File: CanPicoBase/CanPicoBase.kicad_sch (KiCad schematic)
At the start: 17 parts, among them J1 3.50 CBUS, J2 5V select, J3 Grove 2mm, J4 Conn_01x20_Male, J5 Conn_01x20_Male, Q1 DMG2305UX-7, U1 AMS1117-5.0, U2 AMS1117-3.3, U3 Pico

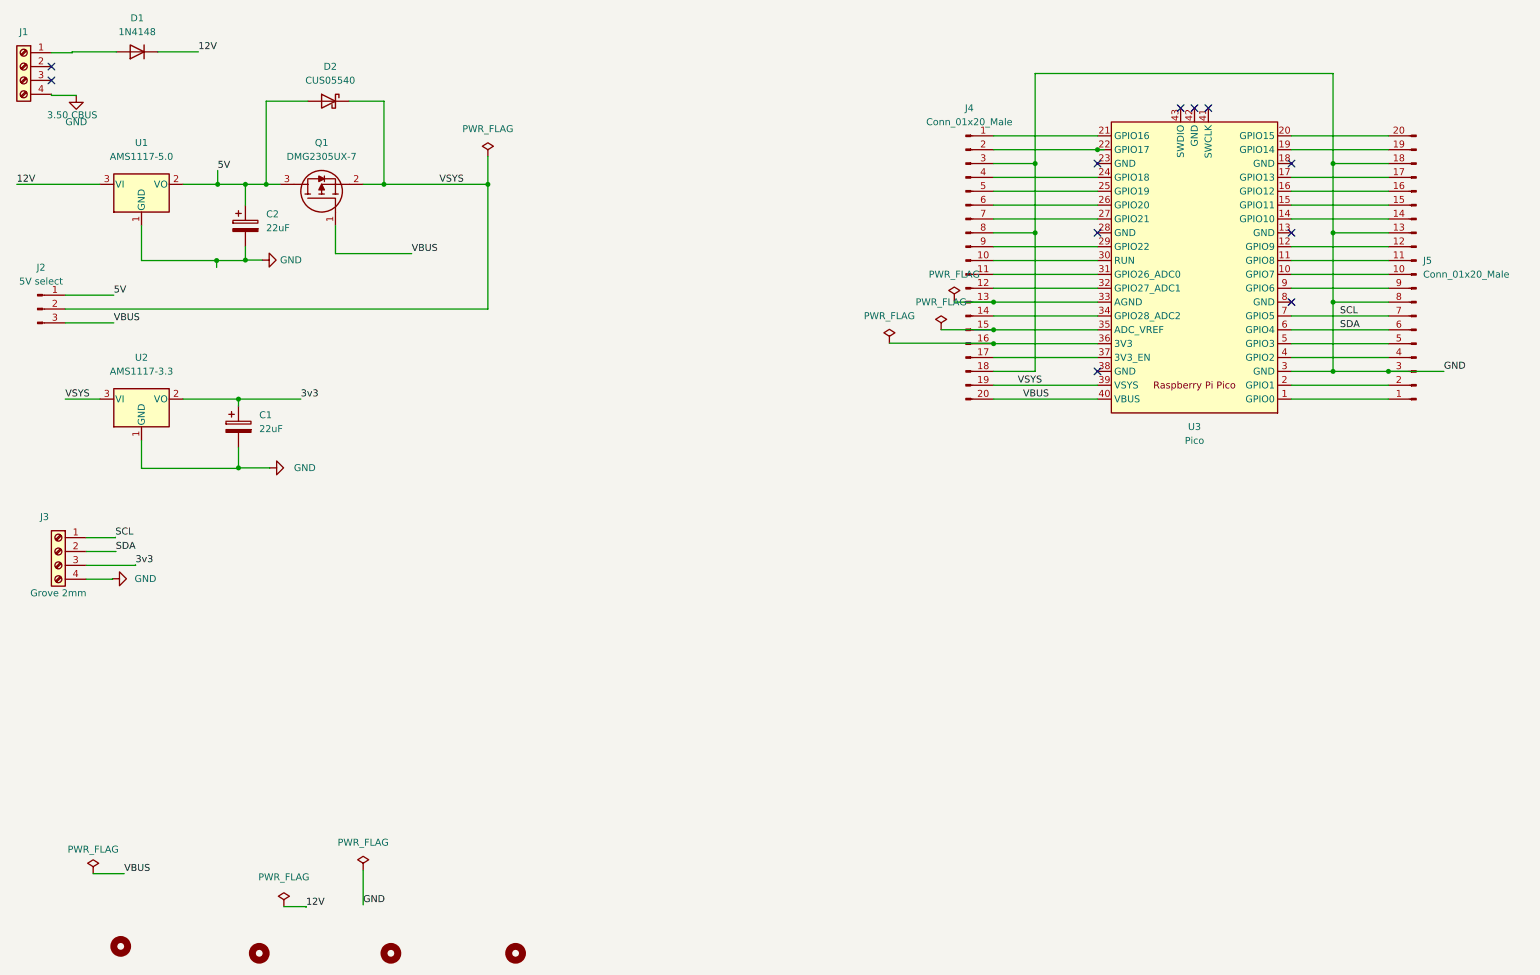
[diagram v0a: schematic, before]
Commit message: 08/09/25 13:36 Titan.local
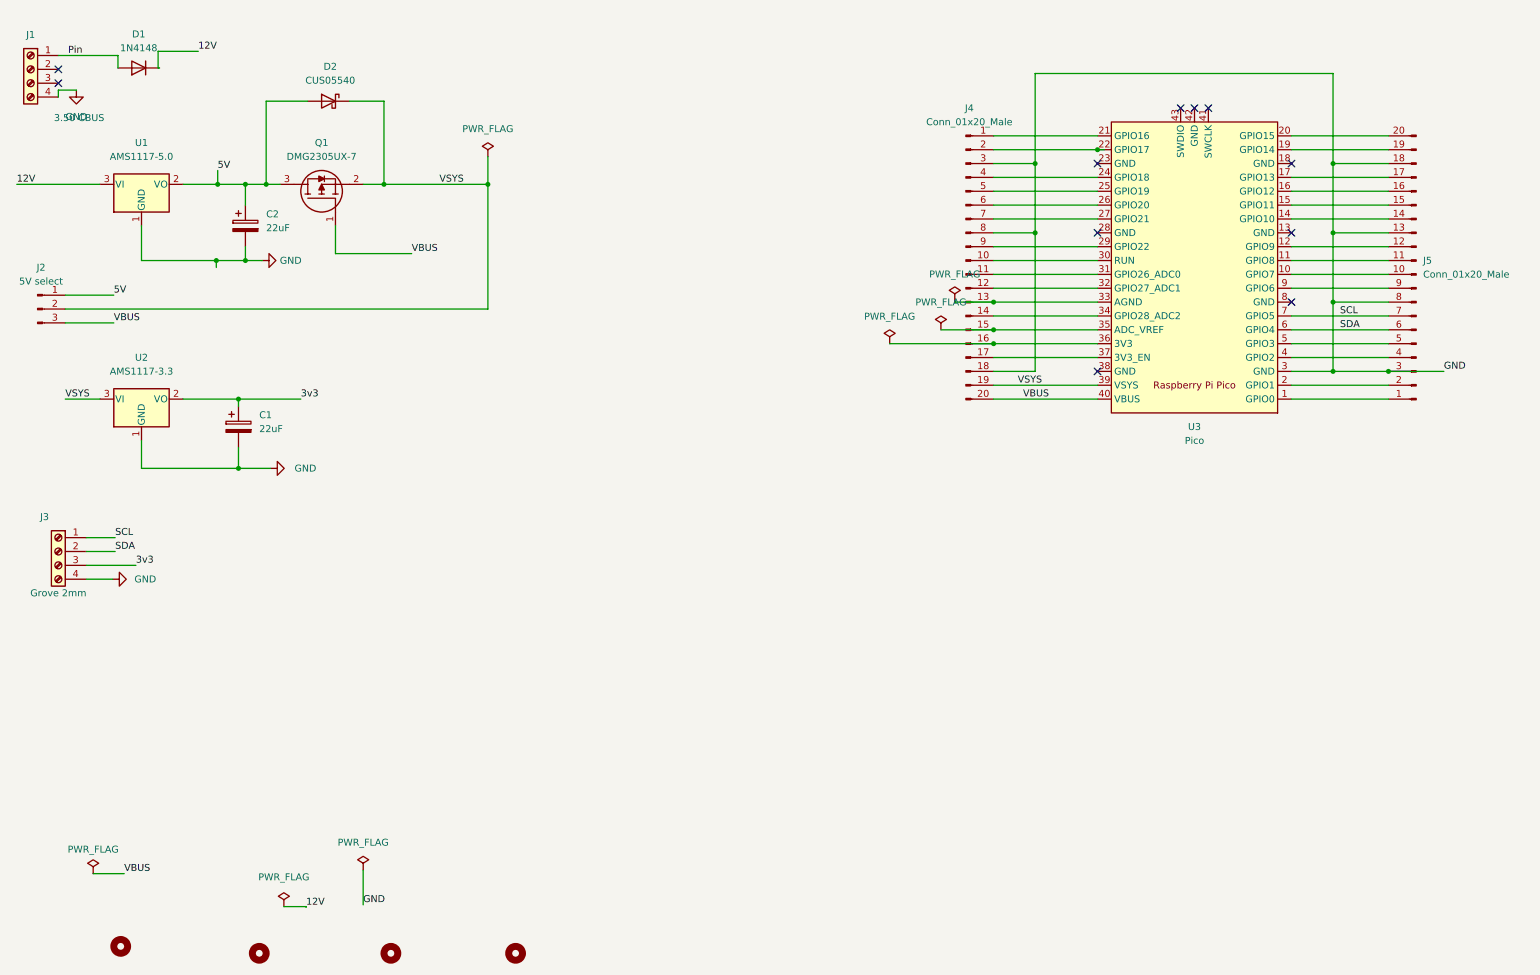
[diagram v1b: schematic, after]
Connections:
- net Pin: now reaches D1.2 (A), J1.1 (Pin_1)
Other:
- moved on the sheet: D1, J1
